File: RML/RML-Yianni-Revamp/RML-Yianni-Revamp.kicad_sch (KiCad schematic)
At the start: 40 parts, among them J1 Tractive, J3 SAMMY-6PIN, Q1 NMOS, Q2 NMOS, U1 LM397, U2 SFH617A-1, U3 LM1117DT-5.0, U4 74AHC1G02, U5 LM555xM

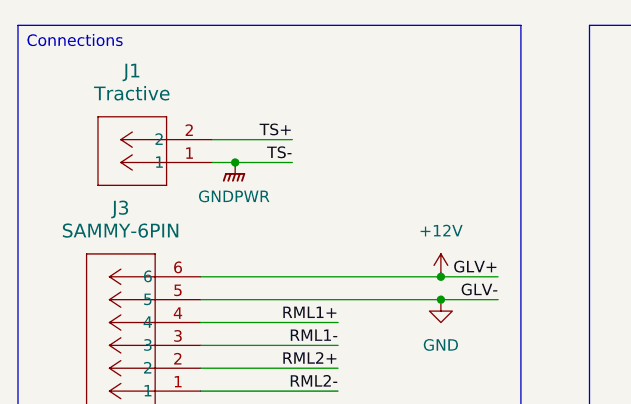
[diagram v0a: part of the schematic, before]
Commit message: Molex Microfit
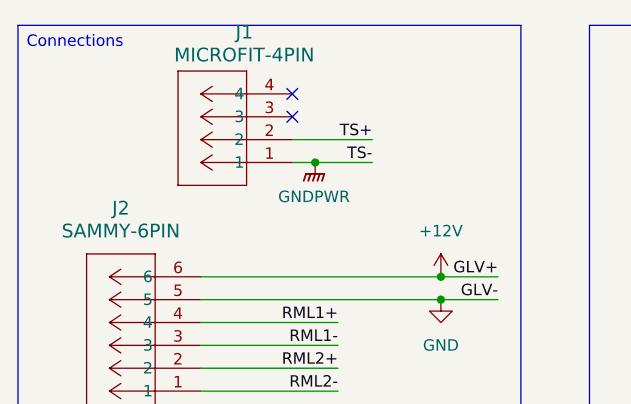
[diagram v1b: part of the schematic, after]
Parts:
- removed J1: Tractive, BSPD:SAMMY-2PIN, symbol BSPD:SAMMY-2PIN
- added J1: MICROFIT-4PIN, RML:MICROFIT-4PIN, symbol RML:MICROFIT-4PIN
- renumbered J3 to J2
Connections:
- net GNDPWR: now also J1.1
- net TS+: now also J1.2
- no-connect marks 3 -> 5
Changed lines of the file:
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@@
 	)
 	(junction
-		(at 39.37 30.48)
+		(at 48.26 30.48)
 		(diameter 0)
 		(color 0 0 0 0)
@@
 	)
 	(no_connect
+		(at 45.72 22.86)
+	)
+	(no_connect
+		(at 45.72 25.4)
+	)
+	(no_connect
 		(at 135.89 31.75)
 	)
@@
 	(wire
 		(pts
-			(xy 36.83 30.48) (xy 39.37 30.48)
+			(xy 45.72 30.48) (xy 48.26 30.48)
 		)
 		(stroke
@@
 	(wire
 		(pts
-			(xy 36.83 27.94) (xy 45.72 27.94)
+			(xy 45.72 27.94) (xy 54.61 27.94)
 		)
 		(stroke
@@
 	(wire
 		(pts
-			(xy 39.37 30.48) (xy 45.72 30.48)
+			(xy 48.26 30.48) (xy 54.61 30.48)
 		)
 		(stroke
@@
 	)
 	(label "TS+"
-		(at 45.72 27.94 180)
+		(at 54.61 27.94 180)
 		(effects
 			(font
@@
 	)
 	(label "TS-"
-		(at 45.72 30.48 180)
+		(at 54.61 30.48 180)
 		(effects
 			(font
@@
 		(dnp no)
 		(fields_autoplaced yes)
-		(property "Reference" "J3"
+		(property "Reference" "J2"
 			(at 26.67 35.56 0)
 			(effects
@@
 			(project ""
 				(path "/6fc260e6-9c33-4f6e-9221-b841b900d5e4"
-					(reference "J3")
+					(reference "J2")
 					(unit 1)
 				)
@@
 	)
 	(symbol
-		(lib_id "BSPD:SAMMY-2PIN")
-		(at 36.83 30.48 180)
-		(unit 1)
-		(exclude_from_sim no)
-		(in_bom yes)
-		(on_board yes)
-		(dnp no)
-		(fields_autoplaced yes)
-		(property "Reference" "J1"
-			(at 27.94 20.32 0)
-			(effects
-				(font
-					(size 1.524 1.524)
-				)
-			)
-		)
-		(property "Value" "Tractive"
-			(at 27.94 22.86 0)
-			(effects
-				(font
-					(size 1.524 1.524)
-				)
-			)
-		)
-		(property "Footprint" "BSPD:SAMMY-2PIN"
-			(at 28.448 24.13 0)
-			(effects
-				(font
-					(size 1.27 1.27)
-					(italic yes)
-				)
-				(hide yes)
-			)
-		)
-		(property "Datasheet" "https://www.molex.com/en-us/products/part-detail-pdf/1053131202?display=pdf"
-			(at 24.384 21.336 0)
-			(effects
-				(font
-					(size 1.27 1.27)
-					(italic yes)
-				)
-				(hide yes)
-			)
-		)
-		(property "Description" ""
-			(at 36.83 30.48 0)
-			(effects
-				(font
-					(size 1.27 1.27)
-				)
-				(hide yes)
-			)
-		)
-		(pin "2"
-		)
-		(pin "1"
-		)
-		(instances
-			(project ""
-				(path "/6fc260e6-9c33-4f6e-9221-b841b900d5e4"
-					(reference "J1")
-					(unit 1)
-				)
-			)
-		)
-	)
-	(symbol
 		(lib_id "Device:R_US")
 		(at 134.62 107.95 0)
@@
 	(symbol
 		(lib_id "power:GNDPWR")
-		(at 39.37 30.48 0)
+		(at 48.26 30.48 0)
 		(unit 1)
 		(exclude_from_sim no)
@@
 		(fields_autoplaced yes)
 		(property "Reference" "#PWR01"
-			(at 39.37 35.56 0)
+			(at 48.26 35.56 0)
 			(effects
 				(font
@@
 		)
 		(property "Value" "GNDPWR"
-			(at 39.243 34.29 0)
+			(at 48.133 34.29 0)
 			(effects
 				(font
@@
 		)
 		(property "Footprint" ""
-			(at 39.37 31.75 0)
+			(at 48.26 31.75 0)
 			(effects
 				(font
@@
 		)
 		(property "Datasheet" ""
-			(at 39.37 31.75 0)
+			(at 48.26 31.75 0)
 			(effects
 				(font
@@
 		)
 		(property "Description" "Power symbol creates a global label with name \"GNDPWR\" , global ground"
-			(at 39.37 30.48 0)
+			(at 48.26 30.48 0)
 			(effects
 				(font
@@
 					(unit 1)
 				)
+			)
+		)
+	)
+	(symbol
+		(lib_id "RML:MICROFIT-4PIN")
+		(at 45.72 30.48 180)
+		(unit 1)
+		(exclude_from_sim no)
+		(in_bom yes)
+		(on_board yes)
+		(dnp no)
+		(property "Reference" "J1"
+			(at 40.386 16.002 0)
+			(effects
+				(font
+					(size 1.524 1.524)
+				)
+			)
+		)
+		(property "Value" "MICROFIT-4PIN"
+			(at 40.386 18.542 0)
+			(effects
+				(font
+					(size 1.524 1.524)
+				)
+			)
+		)
+		(property "Footprint" "RML:MICROFIT-4PIN"
+			(at 45.72 30.48 0)
+			(effects
+				(font
+					(size 1.27 1.27)
+					(italic yes)
+				)
+				(hide yes)
+			)
+		)
+		(property "Datasheet" "https://www.molex.com/en-us/products/part-detail-pdf/447640401?display=pdf"
+			(at 45.72 30.48 0)
+			(effects
+				(font
+					(size 1.27 1.27)
+					(italic yes)
+				)
+				(hide yes)
+			)
+		)
+		(property "Description" ""
+			(at 45.72 30.48 0)
+			(effects
+				(font
+					(size 1.27 1.27)
+				)
+				(hide yes)
+			)
+		)
+		(pin "1"
+		)
+		(pin "3"
+		)
+		(pin "4"
+		)
+		(pin "2"
+		)
+		(instances
+			(project ""
+				(path "/6fc260e6-9c33-4f6e-9221-b841b900d5e4"
+					(reference "J1")
+					(unit 1)
+				)
